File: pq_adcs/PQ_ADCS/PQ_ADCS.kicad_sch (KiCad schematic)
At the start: 55 parts, among them J1 CES-110-02-L-S, J10 Pico-Clasp_01x09, J11 Pico-Clasp_01x15, J12 CES-102-02-L-S, J2 CES-110-02-L-S, J3 CES-110-02-L-S, J4 CES-110-02-L-S, J5 Pico-Clasp_01x03, J6 Pico-Clasp_01x10, J7 Pico-Clasp_01x10, J8 Pico-Clasp_01x10, J9 Pico-Clasp_01x10, U1 LPV542, U2 LPV542, U3 LPV542, U4 IIM-42652, U5 BD2606MVV, U6 TMUX1108RSVR, U7 TCN75AVOA713

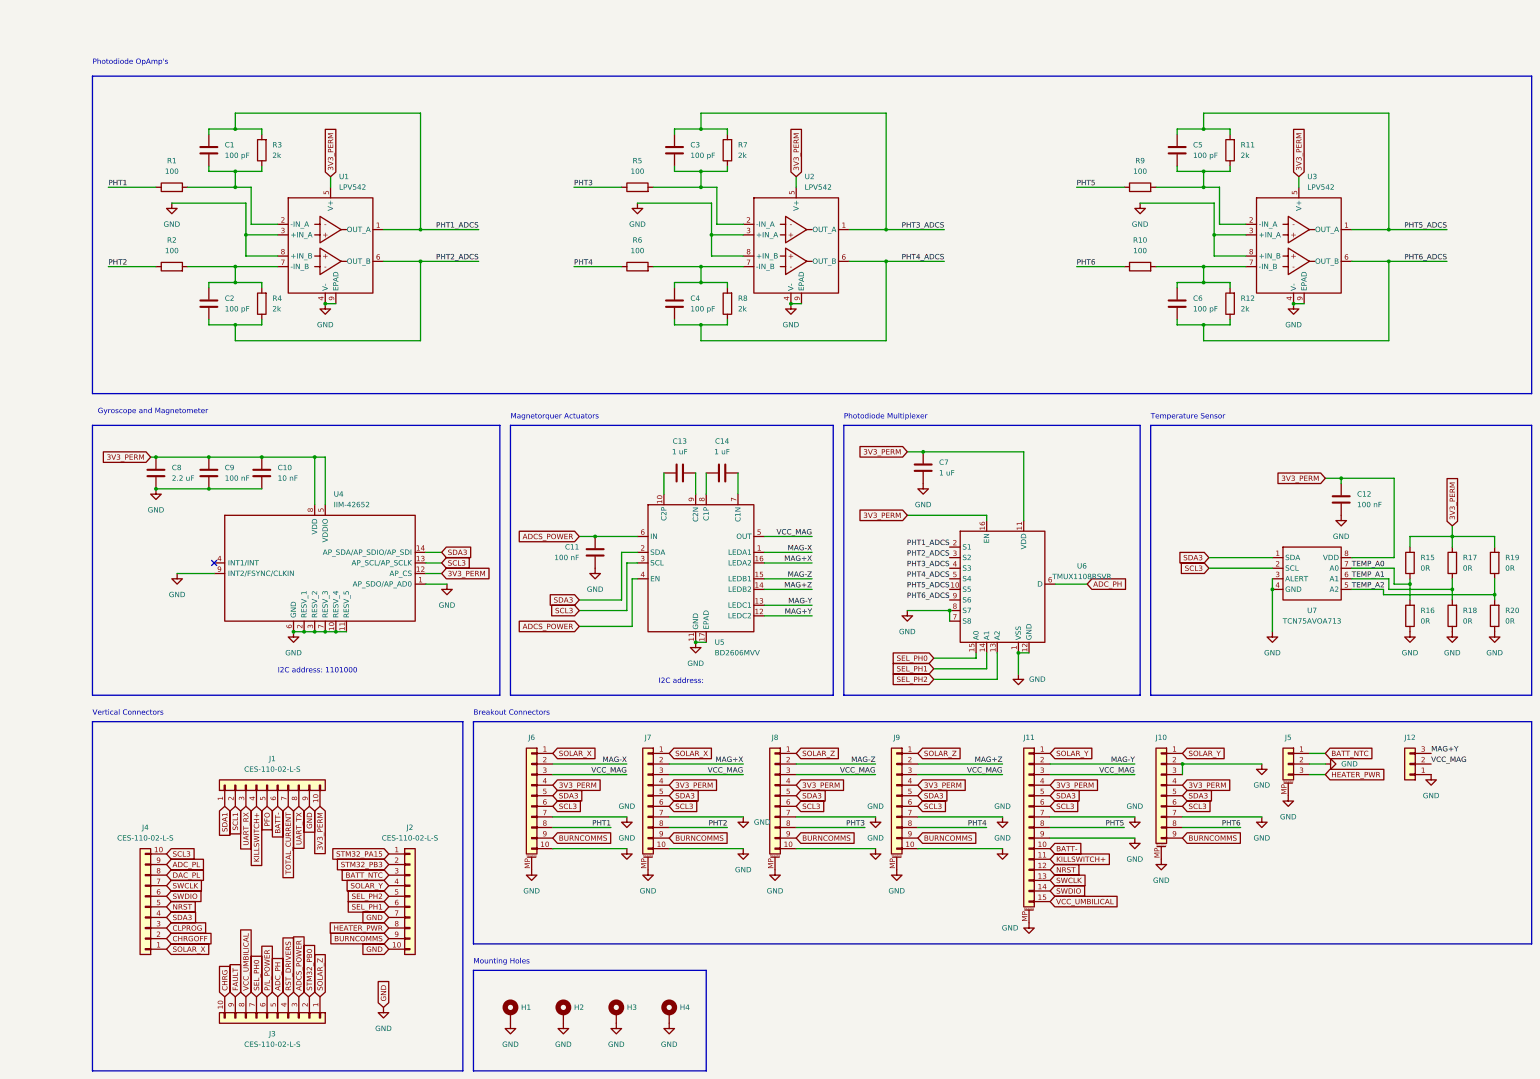
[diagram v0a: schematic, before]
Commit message: document formating
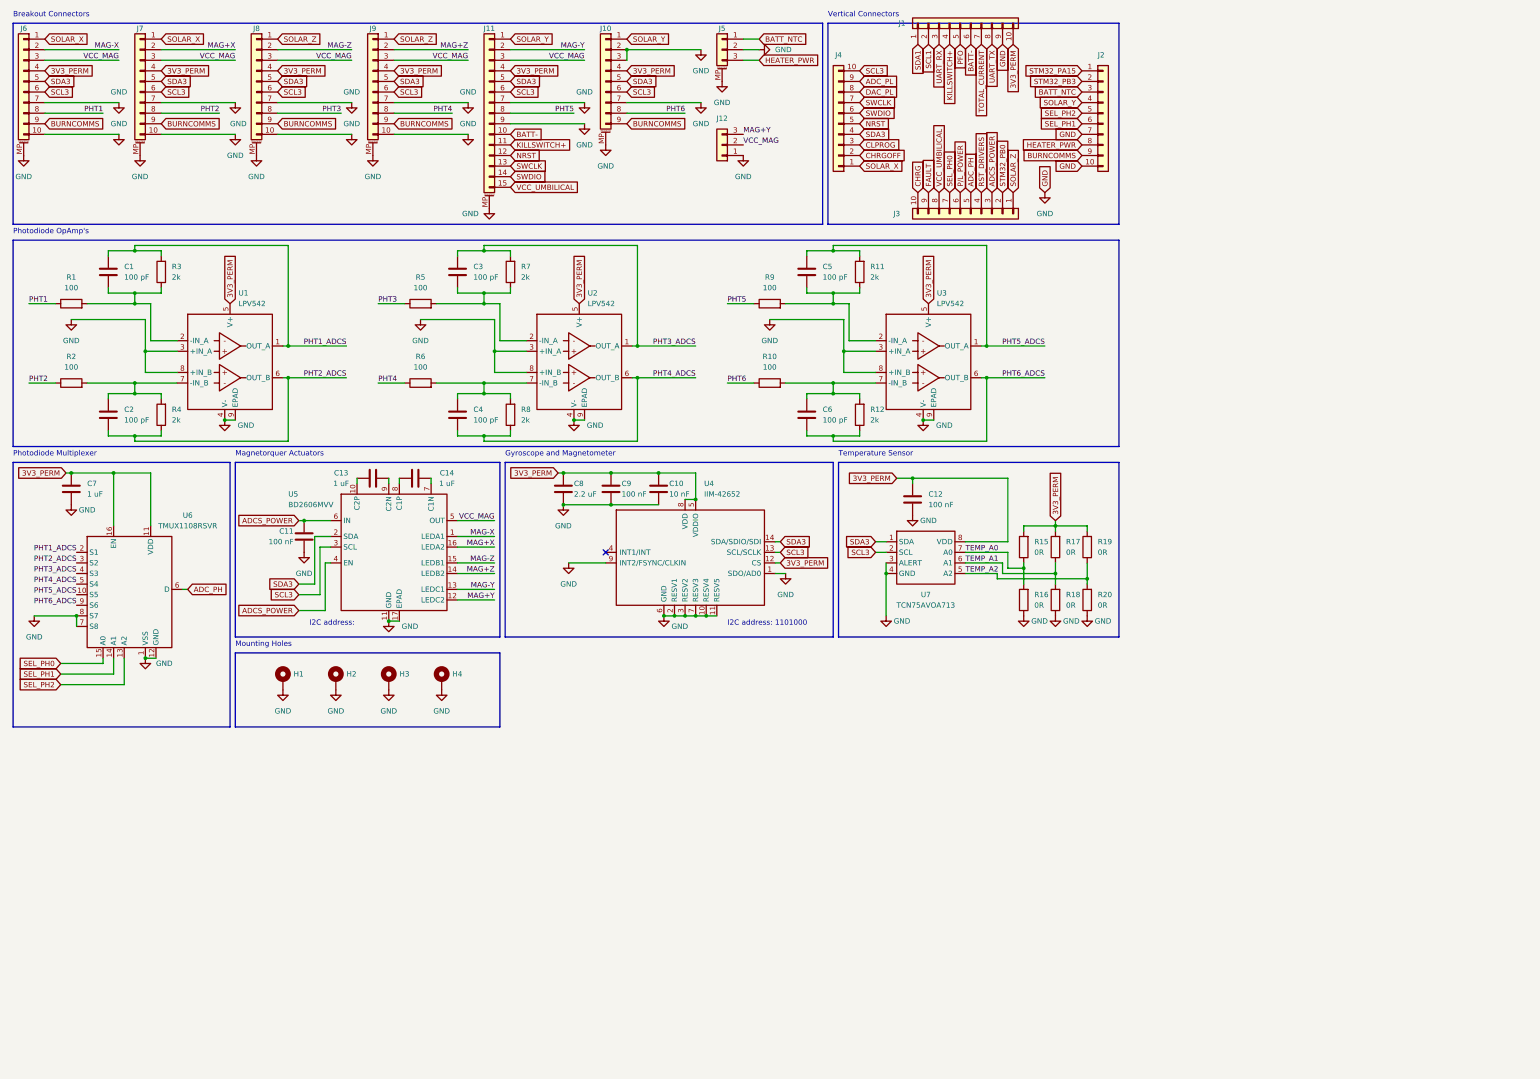
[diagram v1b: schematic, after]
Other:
- company: (none) -> NanoSat Lab UPC
- title: (none) -> ADCS subsyetm schematic
- moved on the sheet: C1, C10, C11, C12, C13, C14, C2, C3, C4, C5, C6, C7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
